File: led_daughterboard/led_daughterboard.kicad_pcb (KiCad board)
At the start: 2 copper layers, 25.4 x 83.8 mm, 12 parts, among them J1 STM32 Black Pill L, J2 STM32 Black Pill R, J3 Barrel_Jack, J4 INMP441_1, J5 INMP441_2, J6 LED_Out, SW1 SW_Push, U1 SN74LV1T34DBV

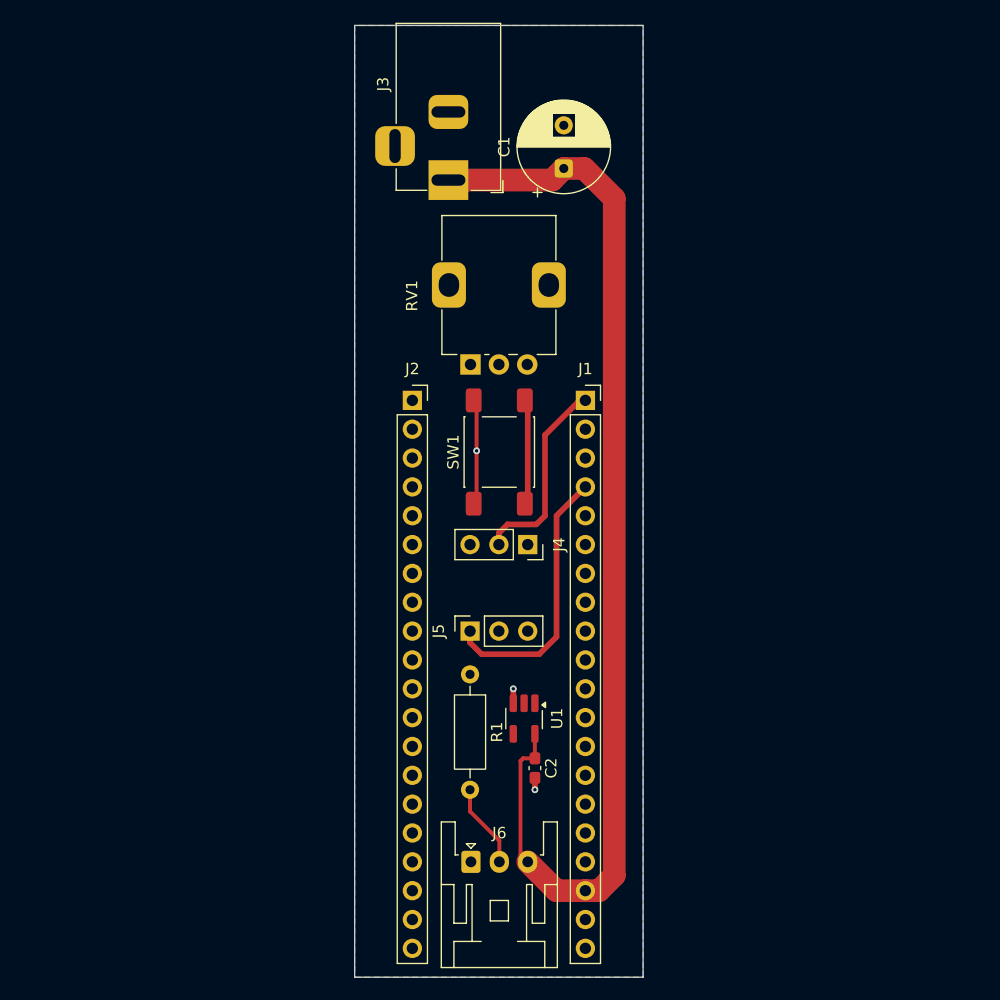
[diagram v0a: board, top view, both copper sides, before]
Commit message: daughterboard tweaks
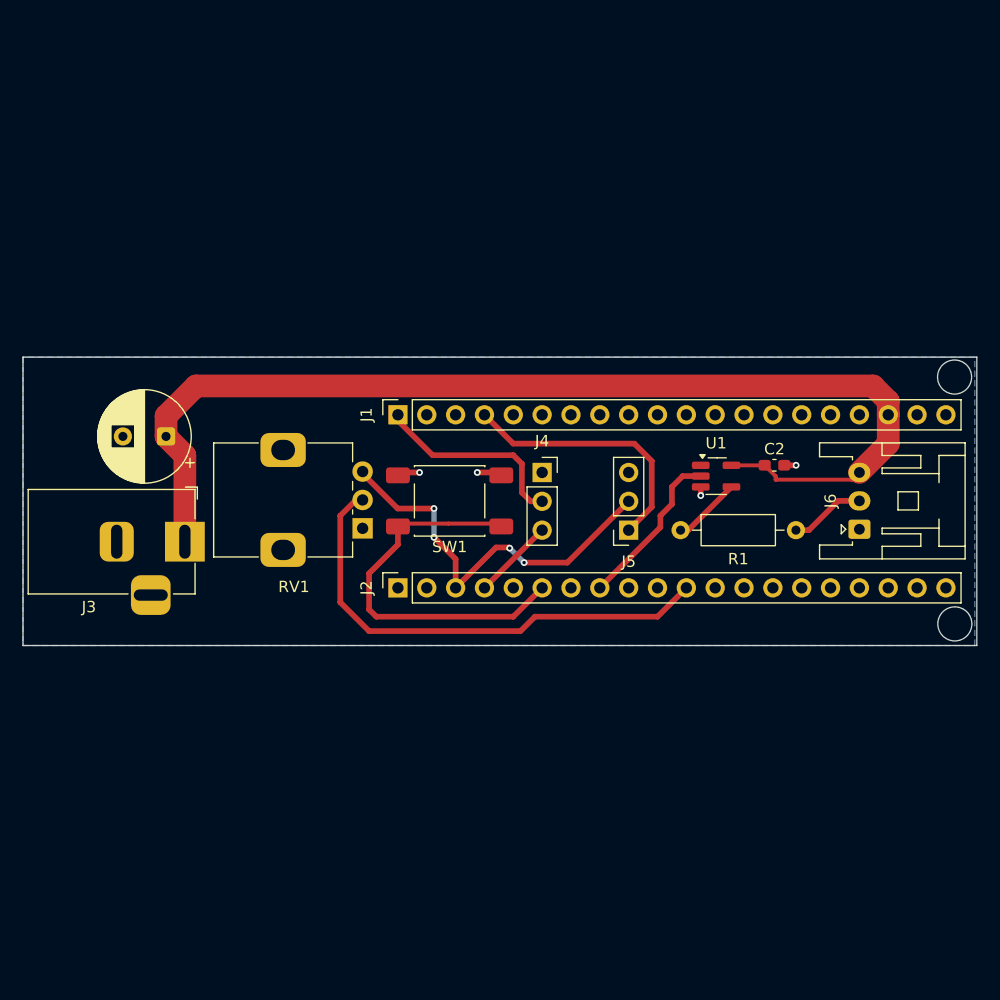
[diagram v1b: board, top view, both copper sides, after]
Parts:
- RV1: value R_Potentiometer -> R_Pot
- moved J6 45.0 mm to (115.6, 62.1), turned to 90 degrees
- moved C1 42.2 mm to (54.5, 54.0), turned to 180 degrees
- moved J3 39.4 mm to (56.2, 63.2), turned to 0 degrees
- moved C2 34.0 mm to (108.1, 56.5), turned to 0 degrees
- moved U1 27.2 mm to (103.0, 57.5), turned to 0 degrees
- moved R1 22.5 mm to (99.8, 62.2), turned to 0 degrees
- moved RV1 17.3 mm to (71.8, 62.1), turned to 180 degrees
- moved J2 16.6 mm to (74.9, 67.3), turned to 90 degrees
- moved J5 16.6 mm to (95.2, 62.2), turned to 180 degrees
- moved J1 16.6 mm to (74.9, 52.1), turned to 90 degrees
- moved J4 6.48 mm to (87.6, 57.1), turned to 0 degrees
- moved SW1 6.14 mm to (79.5, 59.7), turned to 180 degrees
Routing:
- net /A4_Pot: track 0.00 -> 43.2 mm
- net +3.3V: track 0.00 -> 34.9 mm, vias 0 -> 4
- net /B1_Button: track 9.40 -> 34.3 mm, vias 1 -> 0
- net /A7_LED: track 0.00 -> 14.5 mm
- net /B10_I2S2_CK: track 0.00 -> 7.18 mm
- net Net-(U1-Y): track 0.00 -> 6.06 mm
- net GND: track 11.4 -> 6.03 mm, vias 2 -> 4
- net +5V: track 97.7 -> 96.6 mm
- net Net-(J6-Pin_2): track 7.42 -> 6.66 mm
- net /B15_I2S2_SD: track 23.9 -> 23.4 mm
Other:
- board size 25.4 x 83.8 mm -> 84 x 25.4 mm
